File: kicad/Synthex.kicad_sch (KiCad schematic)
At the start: 0 parts

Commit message: Prime ovladani ADSR obalky
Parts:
- added C1, C2: C_Polarized, Capacitor_SMD:CP_Elec_4x5.4, symbol Device:C_Polarized
- added C3: 3n3, Capacitor_SMD:C_1206_3216Metric, symbol Device:C
- added R1: 1k, PCM_4ms_Resistor:R_1206_3216Metric, symbol Device:R
- added R2: 22k, symbol Device:R
- added R3: 10k, symbol Device:R
- added R4: 100k, symbol Device:R
- added U1: NE5532AD, PCM_Package_SO_AKL:SO-8_3.9x4.9mm_P1.27mm, symbol PCM_Amplifier_Operational_AKL:NE5532AD
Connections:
- new net: C1.2, R4.2, U1.3 (+)
- new net: C1.1, C3.1, R1.2
- new net: C2.1, R2.2, U1.1
- new net: R2.1, R3.2, U1.2 (-)
- new net +9V: U1.8 (V+)
- new net -9V: U1.4 (V-)
- new net DAC: R1.1
- new net GND: C3.2, R3.1, R4.1
- new net LINE: C2.2
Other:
- note added: "High pass filtr f ≈ 0.16 Hz Blokování DC offsetu R4 = vstupní impedance"
- note added: "Low pass filtr f ≈ 48kHz"

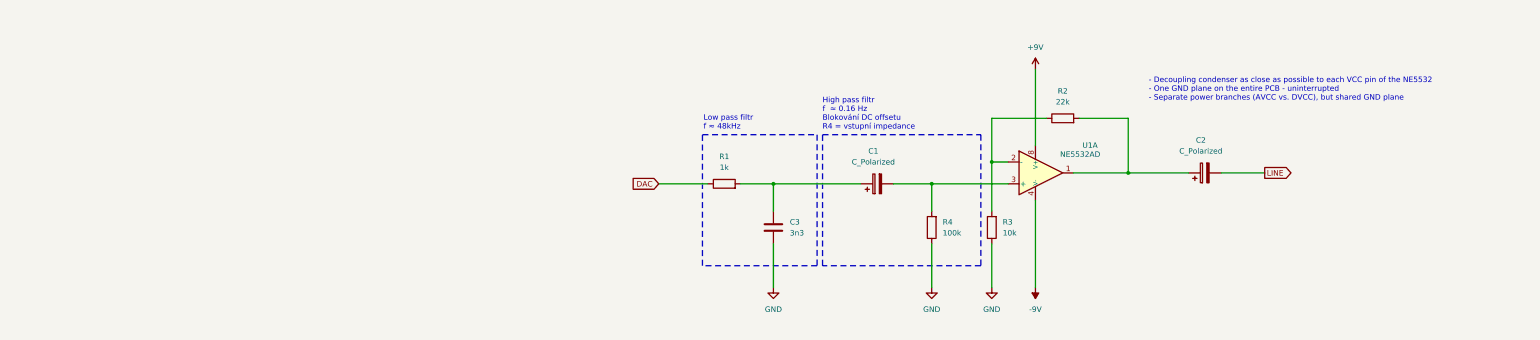
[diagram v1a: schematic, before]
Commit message: pridane schema zapojeni pro DAC a displej
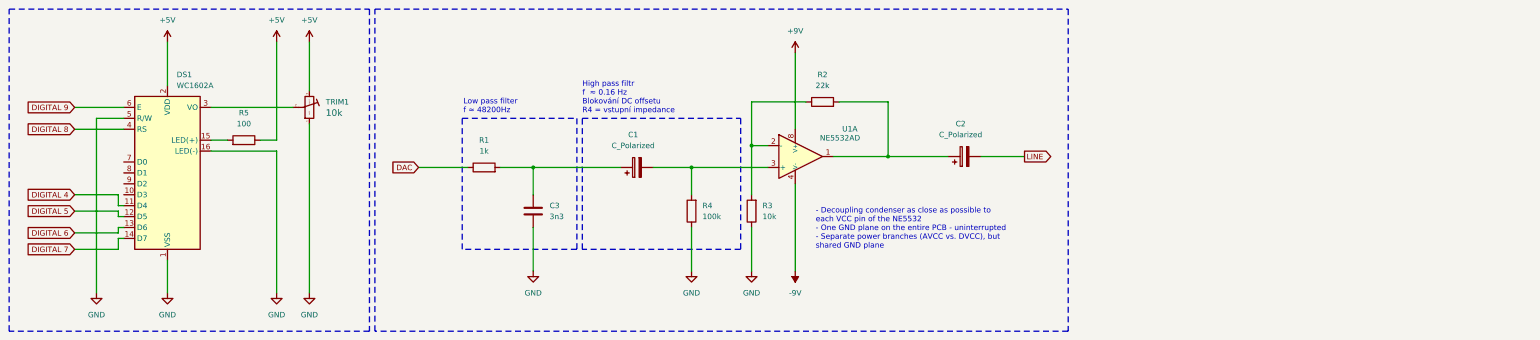
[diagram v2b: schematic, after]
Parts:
- added DS1: WC1602A, Display:WC1602A, symbol Display_Character:WC1602A
- added R5: 100, PCM_4ms_Resistor:R_0603, symbol PCM_Resistor_AKL:R_1206
- added TRIM1: TrimPot_T73YEt_1k, PCM_Potentiometer_THT_AKL:Potentiometer_Bourns_3296W_Vertical, symbol PCM_4ms_Potentiometer:TrimPot_T73YEt_1k
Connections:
- net GND: now also DS1.1 (VSS), DS1.16 (LED(-)), DS1.5 (R/W), TRIM1.1 (Left)
- new net: DS1.3 (VO), TRIM1.2 (Center)
- new net: DS1.15 (LED(+)), R5.1
- new net +5V: DS1.2 (VDD), R5.2, TRIM1.3 (Right)
- new net DIGITAL 4: DS1.11 (D4)
- new net DIGITAL 5: DS1.12 (D5)
- new net DIGITAL 6: DS1.13 (D6)
- new net DIGITAL 7: DS1.14 (D7)
- new net DIGITAL 8: DS1.4 (RS)
- new net DIGITAL 9: DS1.6 (E)
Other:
- note added: "Low pass filter f ≈ 48200Hz"
- note removed: "Low pass filtr f ≈ 48kHz"
- moved on the sheet: C1, C2, C3, R1, R2, R3, R4, U1A
